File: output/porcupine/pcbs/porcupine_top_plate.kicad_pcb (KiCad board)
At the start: 2 copper layers, 129.3 x 113.9 mm, 0 parts

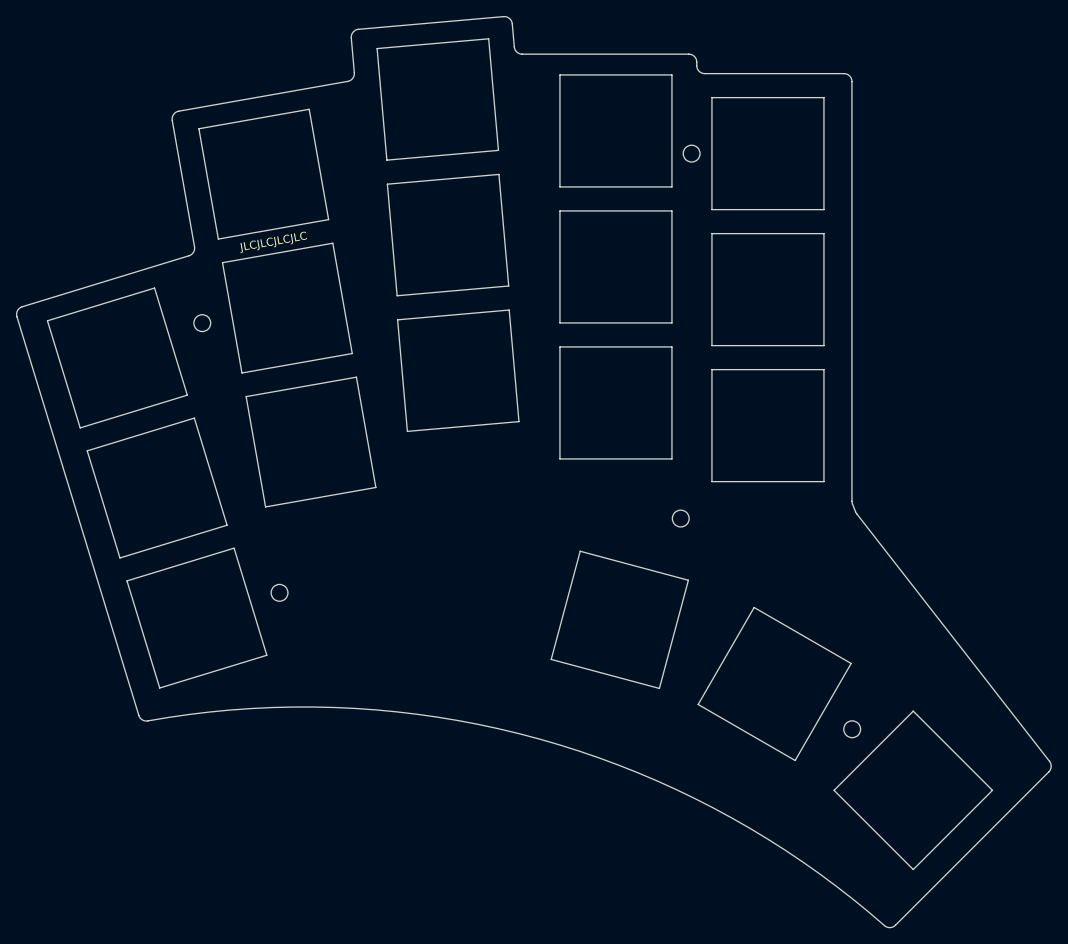
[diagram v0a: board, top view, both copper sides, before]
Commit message: Beschreibung deiner Änderungen
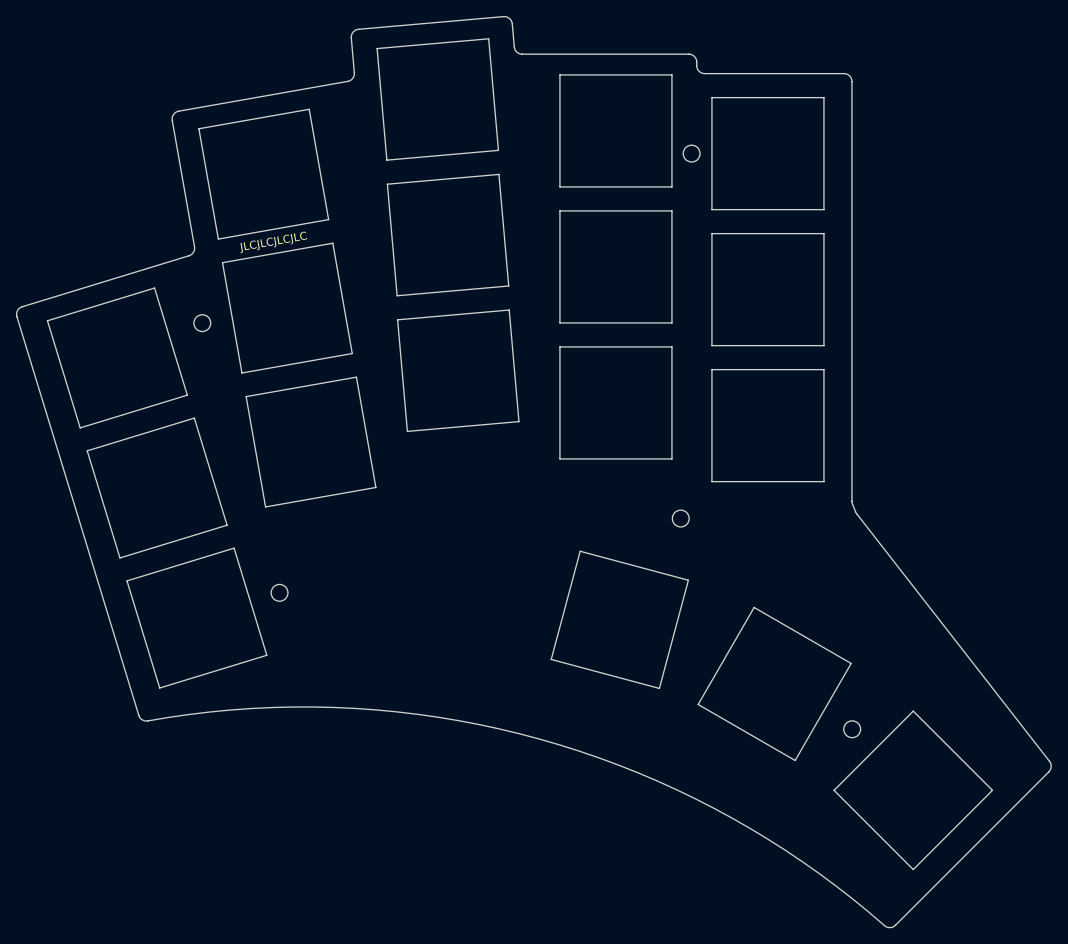
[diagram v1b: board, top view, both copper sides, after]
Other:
- outline, holes or cut-outs redrawn
- net class Default removed
- net class Power removed
